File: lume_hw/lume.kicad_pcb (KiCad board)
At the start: 2 copper layers, 99 x 72 mm, 76 parts, among them SW1 BUTTON, SW2 BUTTON, SW3 BUTTON

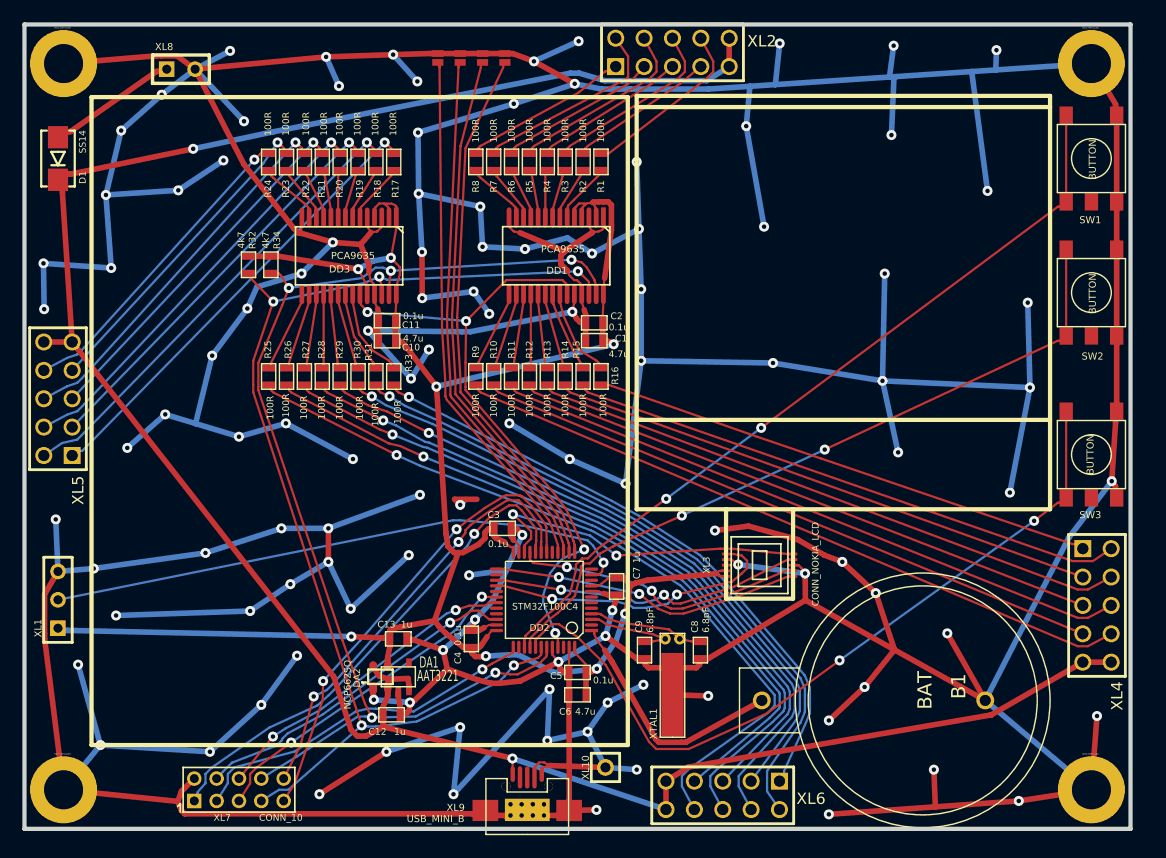
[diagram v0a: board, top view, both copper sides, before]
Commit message: + Lume3 sent to production
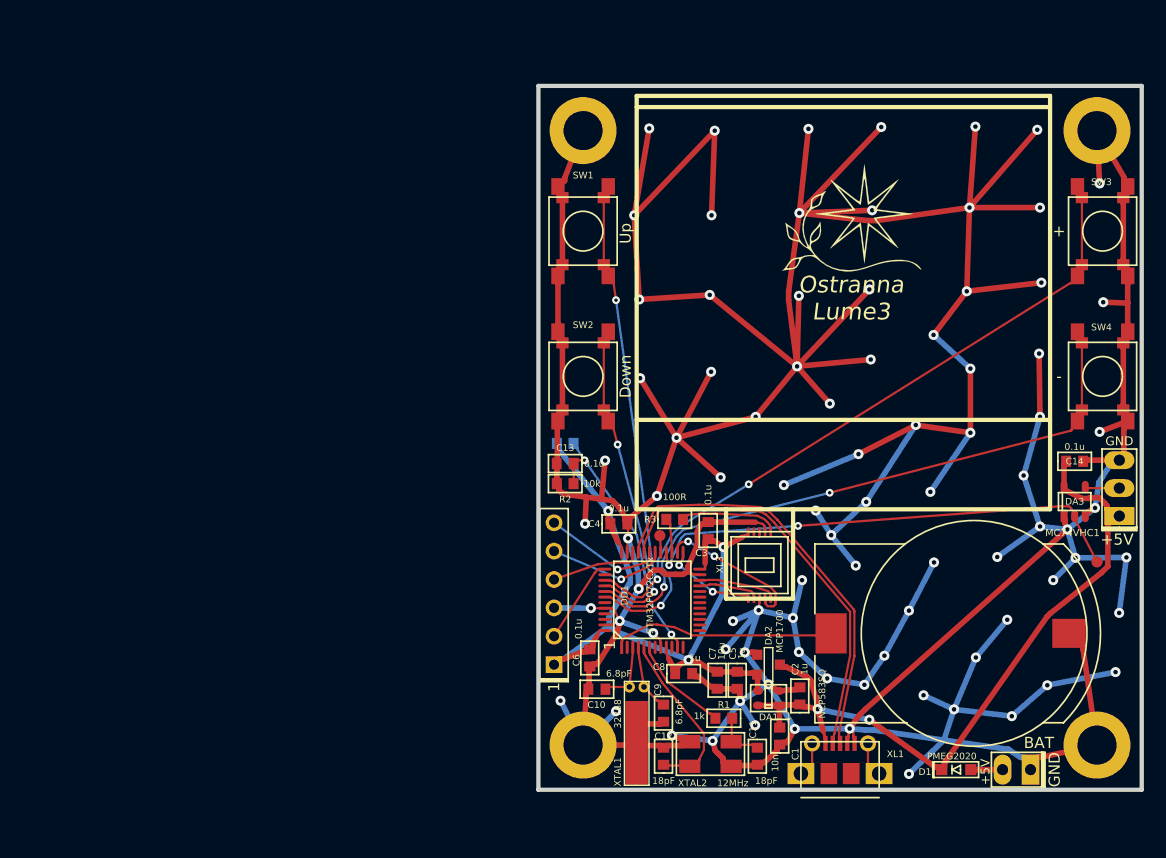
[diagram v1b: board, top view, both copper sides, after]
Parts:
- removed DD2: STM32F100C4, LQFP48
- removed DD3: PCA9635, SSOP28
- removed FU1, FU2, FU3, FU4: SOLDERFUSE, SOLDERFUSE
- removed R10, R11, R12, R13, R14, R15, R16, R17, R18, R19, R20, R21, R22, R23, R24, R25, R26, R27, R28, R29, R30, R31, R33, R4, R5, R6, R7, R8, R9: 100R, RES_0603
- removed R32, R34: 4k7, RES_0603
- removed XL10: CONN_1, SIL-1
- removed XL5, XL6: CONN_10, DIL2x5
- removed XL7: CONN_10, CONN_2MM_2X5
- removed XL9: USB_MINI_B, USB_KMMX_ABSMT5SG_30TR
- added C14: 0.1u, Capacitors:CAP_0603, F.Cu at (201.0, 86.6)
- added DA3: MC74VHC1, SOT:SOT23-5, F.Cu at (201.0, 90.2)
- added Logo1: Logo, Pictures:Ostranna_12d7_10d1, F.Cu at (181.0, 64.8)
- added Q1: ALS-PT19-315C, Resistors:RES_0603, B.Cu at (155.4, 85.0)
- added SW4: BUTTON, BtnsSwitches:BTN_6x6_4x4, F.Cu at (203.5, 79.0)
- added TP1: TESTPOINT, PCB:TESTPOINT_1MM, F.Cu at (163.9, 93.3)
- added TP2: TESTPOINT, PCB:TESTPOINT_1MM, F.Cu at (203.0, 95.6)
- added XTAL2: 12MHz, Quartz:0503x4-4, F.Cu at (168.4, 112.8)
- B1: footprint BAT_BH810 -> Installation:BATTERY_CH7410
- C1: value 4.7u -> 10n; footprint CAP_0603 -> Capacitors:CAP_0603
- C10: value 4.7u -> 6.8pF; footprint CAP_0603 -> Capacitors:CAP_0603
- C11: value 0.1u -> 18pF; footprint CAP_0603 -> Capacitors:CAP_0603
- C12: value 1u -> 18pF; footprint CAP_0603 -> Capacitors:CAP_0603
- C13: value 1u -> 0.1u; footprint CAP_0603 -> Capacitors:CAP_0603
- C2, C5: value 0.1u -> 1u; footprint CAP_0603 -> Capacitors:CAP_0603
- C3, C4, C9: footprint CAP_0603 -> Capacitors:CAP_0603
- C6: value 4.7u -> 0.1u; footprint CAP_0603 -> Capacitors:CAP_0603
- C7: value 1u -> 10u; footprint CAP_0603 -> Capacitors:CAP_0603
- C8: value 6.8pF -> 1u; footprint CAP_0603 -> Capacitors:CAP_0603
- D1: value SS14 -> PMEG2020; footprint DIODE_SMA_DO214AC -> Diodes:SOD323
- DA1: value AAT3221 -> NCP583SQ; footprint SOT23-5 -> SOT:SC82AB
- DA2: value NCP662SQ -> MCP1700; footprint SC82AB -> SOT:SOT23-3
- DD1: value PCA9635 -> STM32F072CxTx; footprint SSOP28 -> LQFP_TQFP:LQFP48
- HOLE1, HOLE2, HOLE3, HOLE4: footprint Hole3_5_out6mm -> PCB:Hole3_5_out6mm
- R1: value 100R -> 1k; footprint RES_0603 -> Resistors:RES_0603
- R2: value 100R -> 10k; footprint RES_0603 -> Resistors:RES_0603
- R3: footprint RES_0603 -> Resistors:RES_0603
- SW1, SW2, SW3: footprint BUTTON_6x6SMD -> BtnsSwitches:BTN_6x6_4x4
- XL1: value CONN_3 -> USB_MINI_B; footprint SIL-3 -> Connectors:USBmicro_MOLEX_1050170001
- XL2: value CONN_10 -> CONN_6; footprint DIL2x5 -> Connectors:PLS-6
- XL3: footprint CONN_NOKIA_LCD -> Connectors:NOKIA_10PIN
- XL4: value CONN_10 -> CONN_3; footprint DIL2x5 -> Connectors:SLD_3_2D5
- XL8: footprint SIL-2 -> Connectors:SLD_2_2D5
- XTAL1: footprint CRYSTAL_KX26 -> Quartz:KX26
- moved XL8 97.6 mm to (195.8, 114.2), turned to 180 degrees
- moved D1 97.2 mm to (190.4, 114.2), turned to 0 degrees
- moved XL1 72.0 mm to (180.0, 116.0), turned to 0 degrees
- moved XL2 55.8 mm to (154.4, 104.8), turned to 90 degrees
- moved C11 51.2 mm to (172.6, 113.0), turned to 270 degrees
- moved R1 51.0 mm to (169.6, 109.6), turned to 180 degrees
- moved HOLE2 46.9 mm to (157.0, 57.0)
- moved HOLE1 46.7 mm to (157.0, 112.0)
- moved SW2 46.1 mm to (157.0, 79.0), turned to 90 degrees
- moved SW1 46.0 mm to (157.0, 66.0), turned to 90 degrees
- moved C1 39.1 mm to (174.6, 111.2), turned to 90 degrees
- moved C2 38.1 mm to (176.4, 107.6), turned to 90 degrees
- moved C10 36.4 mm to (158.2, 107.0)
- moved DA2 34.8 mm to (173.6, 104.8)
- moved R3 33.5 mm to (165.2, 91.8), turned to 0 degrees
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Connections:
- B1 pad A: N-000087 -> Net-(B1-PadA)
- C1 pad 1: +3.3V -> GND
- C1 pad 2: GND -> +5V
- C10 pad 1: +3.3V -> Net-(C10-Pad1)
- C11 pad 1: +3.3V -> Net-(C11-Pad1)
- C12 pad 1: +5V -> Net-(C12-Pad1)
- C13 pad 1: +3.3V -> /LUM_MEAS
- C2 pad 1: +3.3V -> +5V
- C8 pad 1: N-000044 -> +3.3V
- C9 pad 1: N-000098 -> Net-(C9-Pad1)
- D1 pad A: N-000108 -> Net-(D1-PadA)
- DA1 pad 3: +5V -> +3.3V
- DA1 pad 4: (no net) -> +5V
- DA2 pad 2: +5V -> +3.3V
- DA2 pad 3: +3.3V -> +5V
- DD1 pad 1: GND -> Net-(B1-PadA)
- DD1 pad 11: N-000069 -> /LUM_MEAS
- DD1 pad 14: GND -> Net-(DD1-Pad14)
- DD1 pad 2: +3.3V -> Net-(DD1-Pad2)
- DD1 pad 21: N-000070 -> /LCD_SDA
- DD1 pad 22: N-000072 -> /LCD_XRES
- DD1 pad 23: /LED_OE -> GND
- DD1 pad 24: GND -> +3.3V
- DD1 pad 25: GND -> /LCD_SCLK
- DD1 pad 26: /I2C_SCL -> /LCD_XCS
- DD1 pad 27: /I2C_SDA -> /LCD_BCKLT
- DD1 pad 28: +3.3V -> /WS_CTRL
- DD1 pad 3: GND -> Net-(C10-Pad1)
- DD1 pad 4: +3.3V -> Net-(C9-Pad1)
- DD1 pad 5: +3.3V -> Net-(C12-Pad1)
- DD1 pad 6: N-000063 -> Net-(DD1-Pad6)
- DD1 pad 7: N-000064 -> Net-(DD1-Pad7)
- DD1 pad 8: N-000065 -> GND
- DD1 pad 9: N-000062 -> +3.3V
- R1 pad 1: N-000063 -> Net-(C11-Pad1)
- R1 pad 2: N-000002 -> Net-(DD1-Pad6)
- R2 pad 1: N-000064 -> /LUM_MEAS
- R2 pad 2: N-000013 -> GND
- R3 pad 1: N-000065 -> /LCD_BCKLT
- R3 pad 2: N-000011 -> Net-(R3-Pad2)
- XL1 pad 1: +3.3V -> +5V
- XL1 pad 2: N-000107 -> /D-
- XL1 pad 3: GND -> /D+
- XL2 pad 1: N-000010 -> +3.3V
- XL2 pad 2: N-000003 -> /SWCLK
- XL2 pad 3: N-000001 -> GND
- XL2 pad 4: N-000007 -> /SWDIO
- XL2 pad 5: N-000012 -> /UART_TX
- XL2 pad 6: N-000011 -> /UART_RX
- XL3 pad 6: /LCD_BCKLT -> Net-(R3-Pad2)
- XL3 pad 8: (no net) -> Net-(XL3-Pad8)
- XL4 pad 1: N-000005 -> +5V
- XL4 pad 3: N-000006 -> GND
- XL8 pad 1: N-000108 -> GND
- XL8 pad 2: GND -> Net-(D1-PadA)
- XTAL1 pad 1: N-000098 -> Net-(C10-Pad1)
- XTAL1 pad 2: N-000044 -> Net-(C9-Pad1)
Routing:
- net GND: track 1020.8 -> 662.7 mm, vias 113 -> 88
- net +5V: track 209.8 -> 67.2 mm
- net +3.3V: track 188.5 -> 77.4 mm, vias 8 -> 3
- net /I2C_SCL: track 104.8 -> 0.00 mm, vias 5 -> 0
- net /I2C_SDA: track 104.5 -> 0.00 mm, vias 5 -> 0
- net N-000096: track 68.9 -> 0.00 mm, vias 1 -> 0
- net N-000020: track 65.8 -> 0.00 mm, vias 1 -> 0
- net N-000024: track 64.5 -> 0.00 mm, vias 1 -> 0
- net N-000042: track 62.9 -> 0.00 mm, vias 1 -> 0
- net N-000097: track 62.2 -> 0.00 mm
- net N-000022: track 61.5 -> 0.00 mm, vias 1 -> 0
- net N-000018: track 60.2 -> 0.00 mm, vias 1 -> 0
- net N-000026: track 58.6 -> 0.00 mm, vias 1 -> 0
- net N-000008: track 58.3 -> 0.00 mm
- net N-000009: track 57.4 -> 0.00 mm
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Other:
- board size 99 x 72 mm -> 54 x 63 mm
- net class Default: clearance 0.20066 -> 0.18; trace_width 0.20066 -> 0.18; via_dia 0.89916 -> 0.7; via_drill 0.39878 -> 0.3
- net class Wide: clearance 0.20066 -> 0.2; trace_width 0.50038 -> 0.5; via_dia 0.89916 -> 0.9; via_drill 0.39878 -> 0.4
- rule pad_to_mask_clearance: 0.254 -> 0.1
- rule trace_clearance: 0.20066 -> 0.18
- rule trace_min: 0.18034 -> 0.1
- rule via_min_drill: 0.35052 -> 0.2
- rule via_min_size: 0.8001 -> 0.5
- board text added: "+"
- board text added: "+5V"
- board text added: "-"
- board text added: "BAT"
- board text added: "Down"
- board text added: "GND"
- board text added: "Ostranna Lume3"
- board text added: "Up"
